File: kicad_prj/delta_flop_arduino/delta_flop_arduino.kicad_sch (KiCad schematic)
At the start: 18 parts, among them J1 SCREEN OUTPUT, J2 SD_Card, J3 Power connector, SW1 RotaryEncoder_Switch, SW2 Right, SW3 Left, SW4 Enter, U1 Arduino_Nano

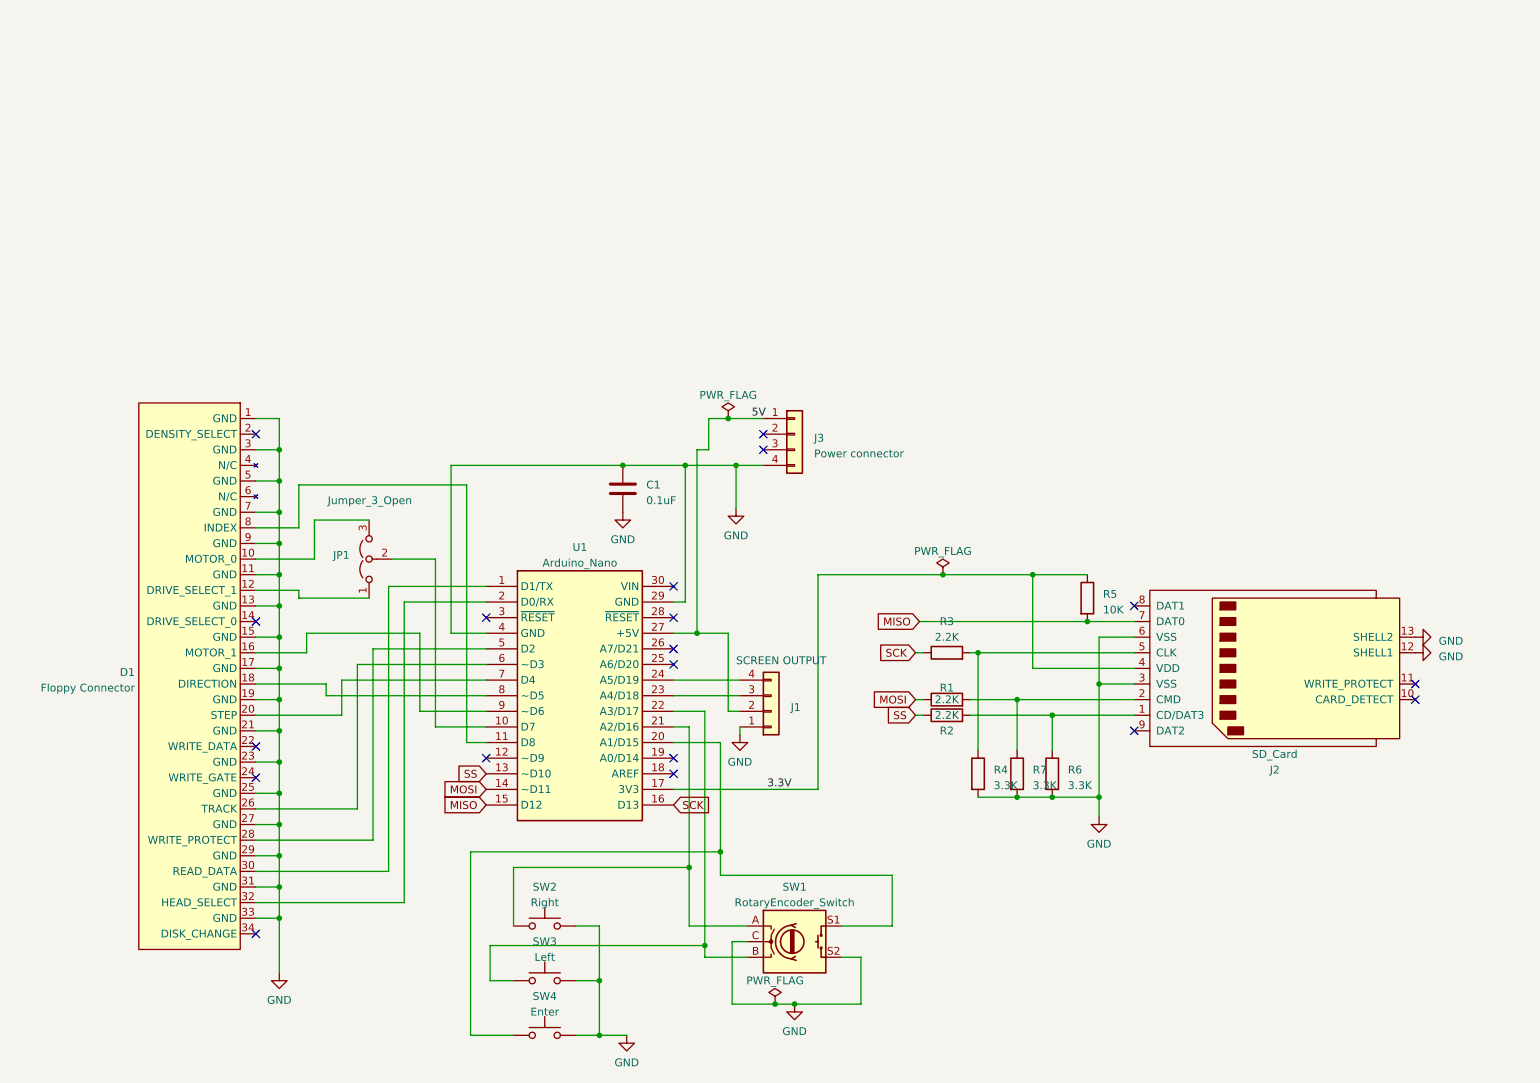
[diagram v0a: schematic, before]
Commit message: New version
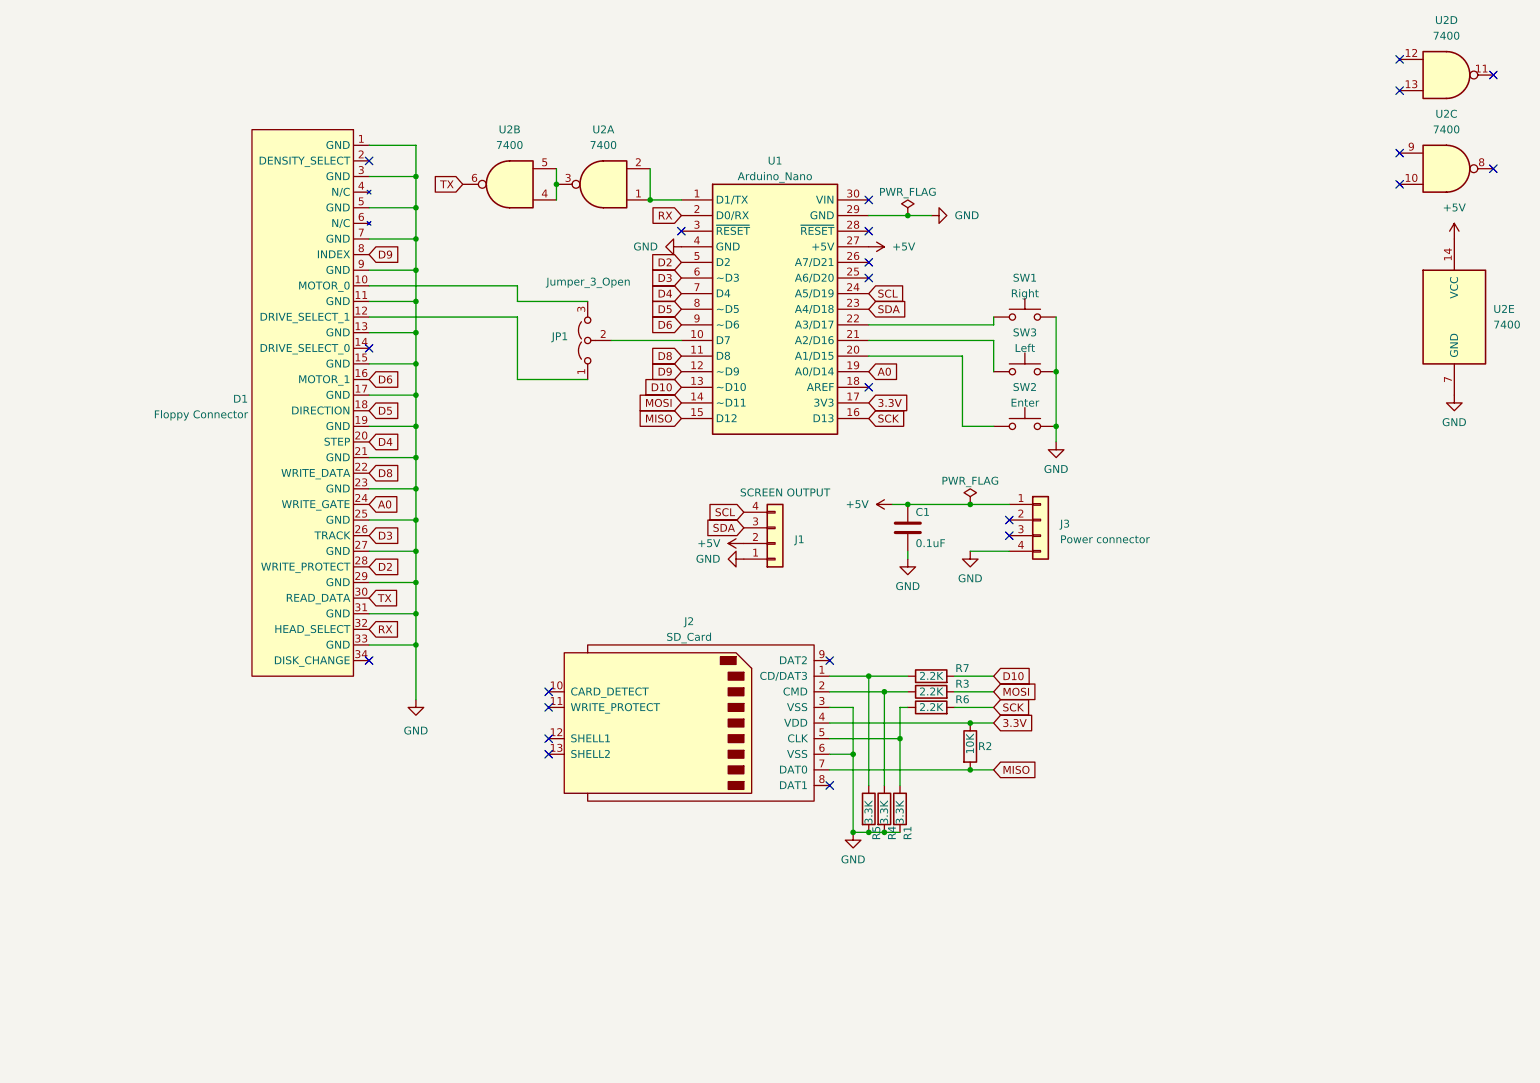
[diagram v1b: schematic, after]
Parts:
- removed C1: 0.1uF, Capacitor_THT:C_Disc_D7.0mm_W2.5mm_P5.00mm, symbol Device:C
- removed D1: Floppy Connector, Connector_IDC:IDC-Header_2x17_P2.54mm_Vertical, symbol delta_flop_pre:34_pin_floppy_convertor
- removed J1: SCREEN OUTPUT, Connector_PinHeader_2.54mm:PinHeader_1x04_P2.54mm_Vertical, symbol delta_flop_pre:Conn_01x04
- removed J2: SD_Card, delta_flop_pre:SDCARD_4UCONN, symbol delta_flop_pre:SD_Card
- removed J3: Power connector, delta_flop_pre:USB-C Power board, symbol Connector_Generic:Conn_01x04
- removed JP1: Jumper_3_Open, Connector_PinHeader_2.54mm:PinHeader_1x03_P2.54mm_Vertical, symbol Jumper:Jumper_3_Open
- removed R1, R2, R3: 2.2K, Resistor_THT:R_Axial_DIN0207_L6.3mm_D2.5mm_P10.16mm_Horizontal, symbol Device:R
- removed R4, R6, R7: 3.3K, Resistor_THT:R_Axial_DIN0207_L6.3mm_D2.5mm_P10.16mm_Horizontal, symbol Device:R
- removed R5: 10K, Resistor_THT:R_Axial_DIN0207_L6.3mm_D2.5mm_P10.16mm_Horizontal, symbol Device:R
- removed SW1: RotaryEncoder_Switch, Rotary_Encoder:RotaryEncoder_Alps_EC11E-Switch_Vertical_H20mm, symbol delta_flop_pre:RotaryEncoder_Switch
- removed SW2: Right, Button_Switch_THT:SW_PUSH_6mm, symbol Switch:SW_Push
- removed SW3: Left, Button_Switch_THT:SW_PUSH_6mm, symbol Switch:SW_Push
- removed SW4: Enter, Button_Switch_THT:SW_PUSH_6mm, symbol Switch:SW_Push
- removed U1: Arduino_Nano, delta_flop_pre:Arduino_Nano, symbol delta_flop_pre:Arduino_Nano
- added C1: 0.1uF, Floppy_emu_footprints:C_Disc_D7.0mm_W2.5mm_P5.00mm, symbol floppy_symbols:C
- added D1: Floppy Connector, Floppy_emu_footprints:IDC-Header_2x17_P2.54mm_Vertical, symbol floppy_symbols:34_pin_floppy_convertor
- added J1: SCREEN OUTPUT, Floppy_emu_footprints:PinHeader_1x04_P2.54mm_Vertical, symbol floppy_symbols:Conn_01x04
- added J2: SD_Card, Floppy_emu_footprints:SDCARD_4UCONN, symbol floppy_symbols:SD_Card
- added J3: Power connector, Floppy_emu_footprints:USB-C Power board, symbol floppy_symbols:Conn_01x04
- added JP1: Jumper_3_Open, Floppy_emu_footprints:PinHeader_1x03_P2.54mm_Vertical, symbol floppy_symbols:Jumper_3_Open
- added R1, R4, R5: 3.3K, Floppy_emu_footprints:R_Axial_DIN0207_L6.3mm_D2.5mm_P10.16mm_Horizontal, symbol floppy_symbols:R
- added R2: 10K, Floppy_emu_footprints:R_Axial_DIN0207_L6.3mm_D2.5mm_P10.16mm_Horizontal, symbol floppy_symbols:R
- added R3, R6, R7: 2.2K, Floppy_emu_footprints:R_Axial_DIN0207_L6.3mm_D2.5mm_P10.16mm_Horizontal, symbol floppy_symbols:R
- added SW1: Right, Floppy_emu_footprints:SW_PUSH_6mm, symbol floppy_symbols:SW_Push
- added SW2: Enter, Floppy_emu_footprints:SW_PUSH_6mm, symbol floppy_symbols:SW_Push
- added SW3: Left, Floppy_emu_footprints:SW_PUSH_6mm, symbol floppy_symbols:SW_Push
- added U1: Arduino_Nano, w_conn_av:Arduino_Nano, symbol floppy_symbols:Arduino_Nano
- added U2: 7400, Floppy_emu_footprints:DIP-14_W7.62mm_Socket_LongPads, symbol floppy_symbols:7400
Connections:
- net 3.3V: now also J2.4 (VDD), R2.1, U1.17 (3V3)
- net GND: now also C1.2, D1.1 (GND), D1.11 (GND), D1.13 (GND), D1.15 (GND), D1.17 (GND), D1.19 (GND), D1.21 (GND), D1.23 (GND), D1.25 (GND), D1.27 (GND), D1.29 (GND), D1.3 (GND), D1.31 (GND), D1.33 (GND), D1.5 (GND), D1.7 (GND), D1.9 (GND), J1.1 (Pin_1), J2.3 (VSS), J2.6 (VSS), J3.4 (Pin_4), R1.2, R4.2, R5.2, SW1.2, SW2.2, SW3.2, U1.29 (GND), U1.4 (GND), U2.7 (GND)
- net MISO: now also J2.7 (DAT0), R2.2, U1.15 (D12)
- net MOSI: now also R3.2, U1.14 (~D11)
- net SCK: now also R6.2, U1.16 (D13)
- new net: J2.5 (CLK), R1.1, R6.1
- new net: J2.1 (CD/DAT3), R5.1, R7.1
- new net: U1.1 (D1/TX), U2.1, U2.2
- new net: JP1.2 (C), U1.10 (D7)
- new net: SW2.1, U1.20 (A1/D15)
- new net: SW3.1, U1.21 (A2/D16)
- new net: SW1.1, U1.22 (A3/D17)
- new net: U2.3, U2.4, U2.5
- new net: J2.2 (CMD), R3.1, R4.1
- new net: D1.10 (MOTOR_0), JP1.3 (B)
- new net: D1.12 (DRIVE_SELECT_1), JP1.1 (A)
- new net +5V: C1.1, J1.2 (Pin_2), J3.1 (Pin_1), U1.27 (+5V), U2.14 (VCC)
- new net A0: D1.24 (WRITE_GATE), U1.19 (A0/D14)
- new net D10: R7.2, U1.13 (~D10)
- new net D2: D1.28 (WRITE_PROTECT), U1.5 (D2)
- new net D3: D1.26 (TRACK), U1.6 (~D3)
- new net D4: D1.20 (STEP), U1.7 (D4)
- new net D5: D1.18 (DIRECTION), U1.8 (~D5)
- new net D6: D1.16 (MOTOR_1), U1.9 (~D6)
- new net D8: D1.22 (WRITE_DATA), U1.11 (D8)
- new net D9: D1.8 (INDEX), U1.12 (~D9)
- new net RX: D1.32 (HEAD_SELECT), U1.2 (D0/RX)
- new net SCL: J1.4 (Pin_4), U1.24 (A5/D19)
- new net SDA: J1.3 (Pin_3), U1.23 (A4/D18)
- new net TX: D1.30 (READ_DATA), U2.6
- no-connect marks 19 -> 23
